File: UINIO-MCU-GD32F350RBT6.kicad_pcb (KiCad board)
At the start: 2 copper layers, 81.5 x 20.3 mm, 39 parts, among them J1 Conn_01x32_Male, J2 Conn_01x32_Male, J3 Conn_01x04_Male, SW1 BOOT0, SW2 NRST, U1 ME6211C33M5G-N, U2 GD32F350RBT6, Y1 32.768KHz, Y2 8MHz

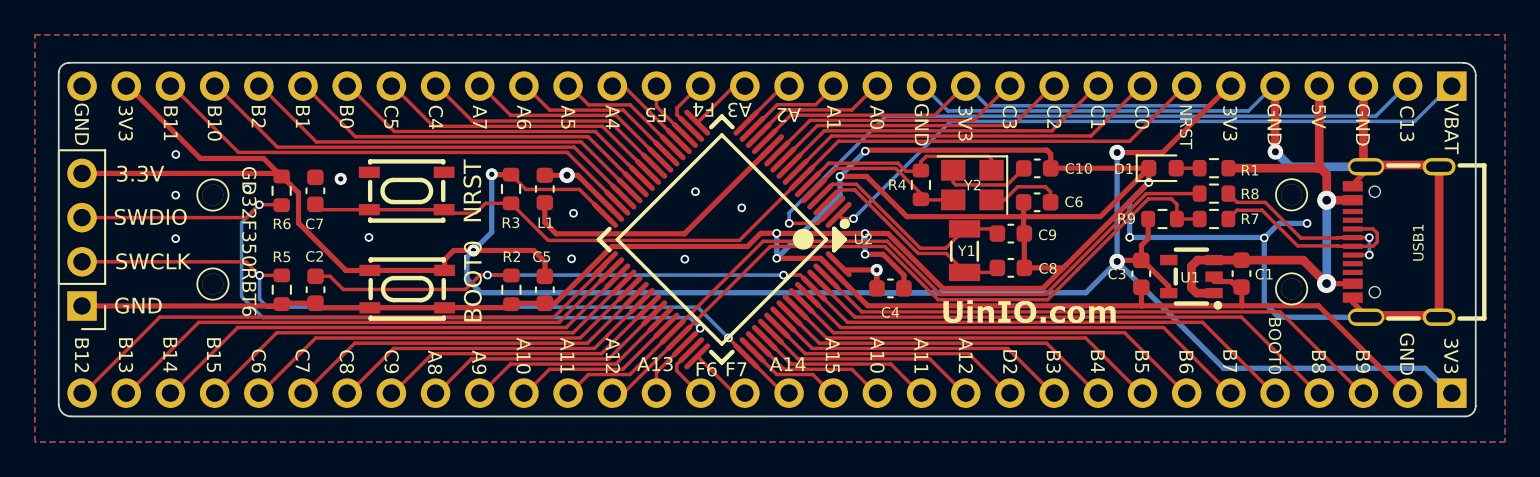
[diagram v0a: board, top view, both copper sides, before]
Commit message: Release UINIO-MCU-GD32F350RBT6 version 1.0.0.
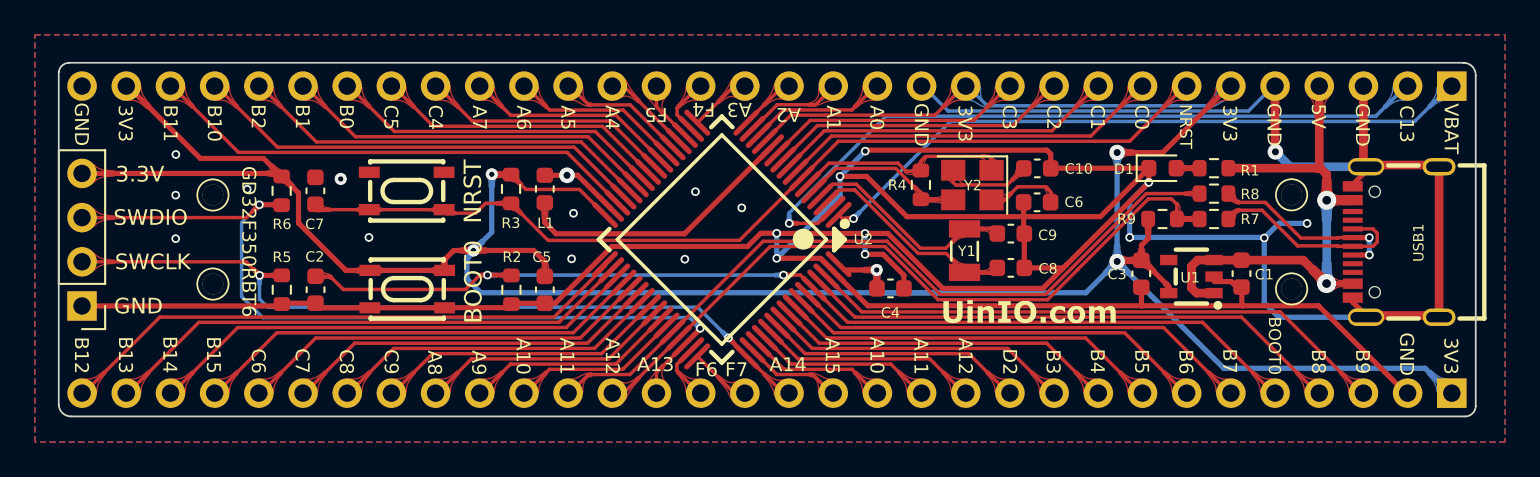
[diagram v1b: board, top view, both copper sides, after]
